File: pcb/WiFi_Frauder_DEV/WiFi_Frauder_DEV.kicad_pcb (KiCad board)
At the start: 2 copper layers, 93.4 x 64.5 mm, 11 parts, among them SW1 BTN_DOWN, SW2 BTN_UP, SW3 BTN_ENTER, U1 ESP32-DevKitC, U2 DM-OLED096-636

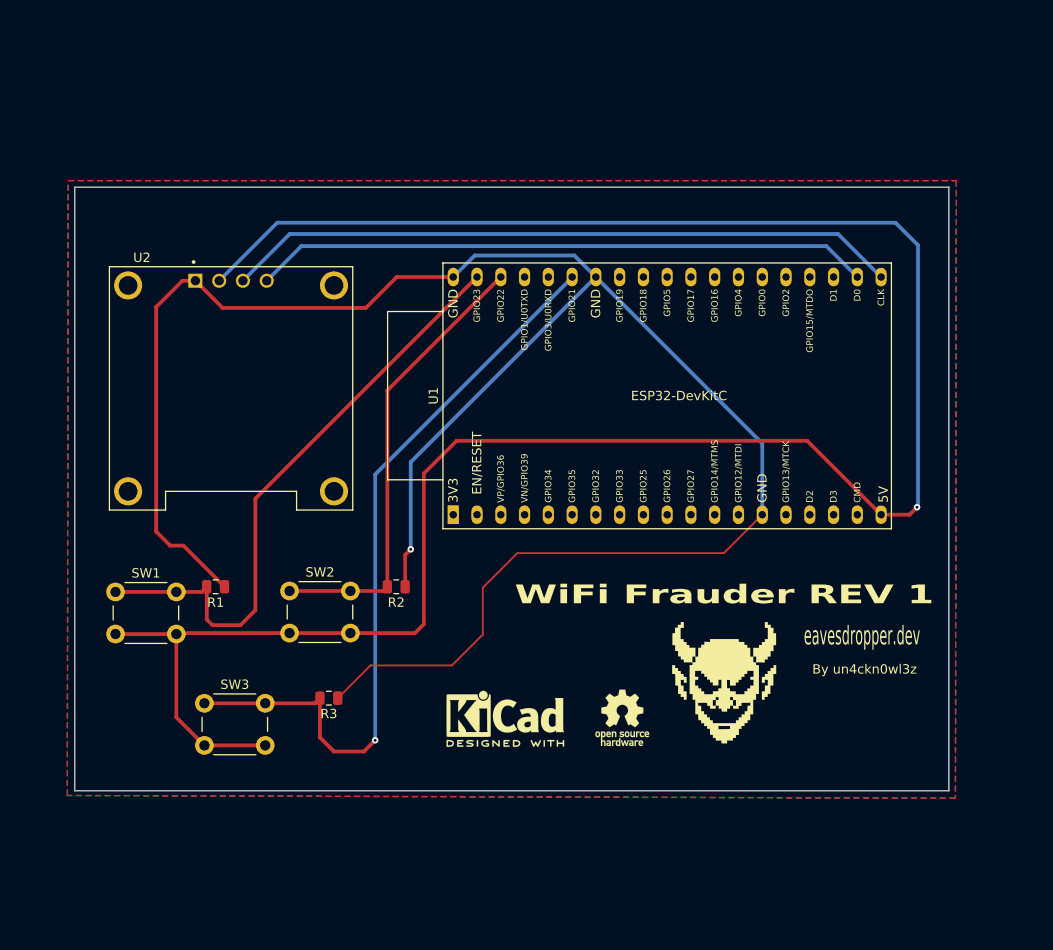
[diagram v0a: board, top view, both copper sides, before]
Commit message: feat: revistion pcb to rev2
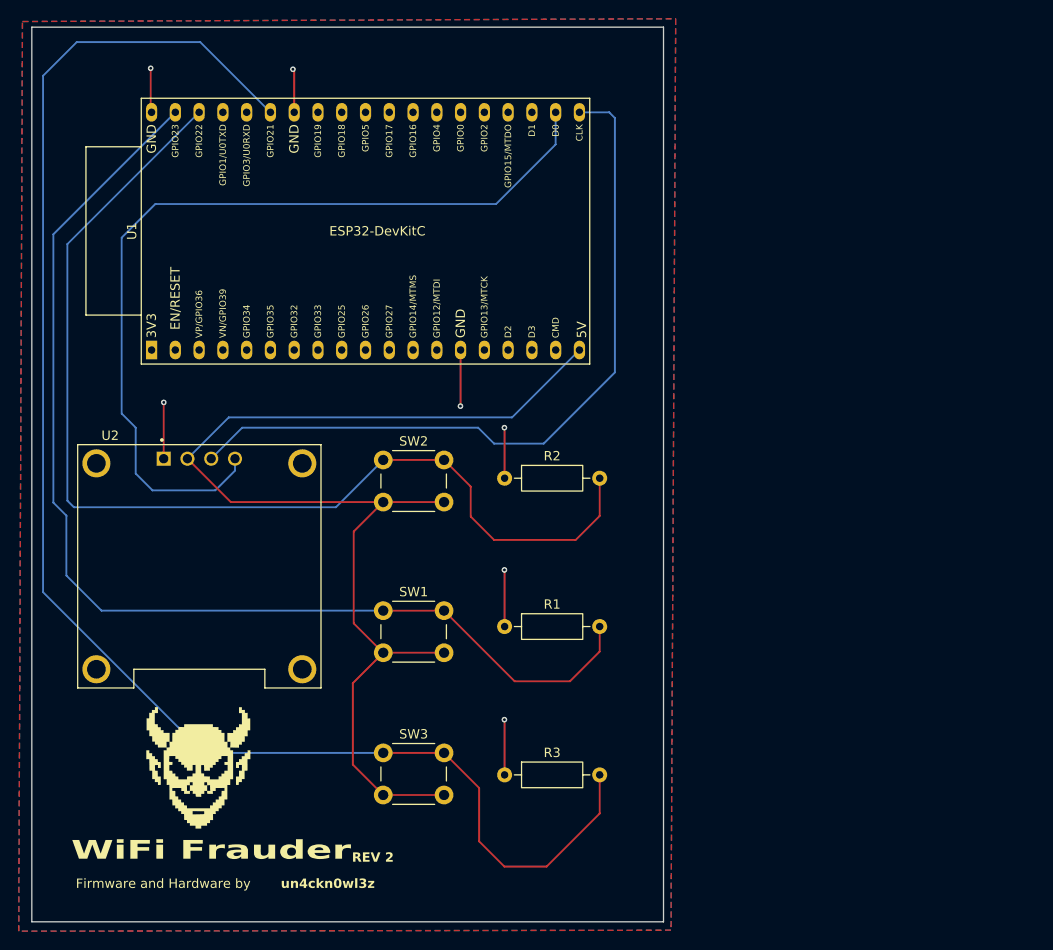
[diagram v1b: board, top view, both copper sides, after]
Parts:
- removed REF**: OSHW-Logo_5.7x6mm_SilkScreen, Symbol:OSHW-Logo_5.7x6mm_SilkScreen
- removed REF**: KiCad-Logo2_5mm_SilkScreen, Symbol:KiCad-Logo2_5mm_SilkScreen
- R1, R2, R3: footprint Capacitor_SMD:C_0805_2012Metric -> Resistor_THT:R_Axial_DIN0207_L6.3mm_D2.5mm_P10.16mm_Horizontal
- moved G*** 56.9 mm to (133.0, 121.6)
- moved U1 36.7 mm to (128.0, 77.1)
- moved R1 31.2 mm to (165.7, 106.7), turned to 0 degrees
- moved SW1 28.7 mm to (152.8, 105.0)
- moved R3 20.5 mm to (165.7, 122.5), turned to 0 degrees
- moved SW3 19.8 mm to (152.8, 120.2)
- moved U2 19.3 mm to (133.1, 100.2)
- moved SW2 17.2 mm to (152.8, 88.8)
- moved R2 16.4 mm to (165.7, 90.8), turned to 0 degrees
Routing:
- net GND: track 217.1 -> 38.8 mm, vias 1 -> 7
- net +5V: track 233.2 -> 125.6 mm, vias 1 -> 0
- net /BTN_ENTER_NET: track 82.0 -> 165.5 mm, vias 1 -> 0
- net /BTN_UP_NET: track 48.8 -> 117.1 mm
- net /BTN_DOWN_NET: track 65.0 -> 121.1 mm
- net /OLED_SDA_NET: track 66.0 -> 93.3 mm
- net /OLED_SCL_NET: track 72.2 -> 79.6 mm
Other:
- board size 93.4 x 64.5 mm -> 67.5 x 95.6 mm
- board text added: "Firmware and Hardware by"
- board text added: "REV 2"
- board text added: "WiFi Frauder"
- board text added: "un4ckn0wl3z"
- board text removed: "By un4ckn0wl3z"
- board text removed: "WiFi Frauder REV 1"
- board text removed: "eavesdropper.dev"
